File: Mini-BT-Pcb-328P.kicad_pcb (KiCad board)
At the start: 2 copper layers, 55 x 35 mm, 51 parts, among them J1 Analog IN, J2 USB_B_Micro, J3 Booster CE, J5 ANT, P1 MYSX_2.6, Q1 FDN338P, Q2 FDN337N, SW2 Reset, SW3 SW_Reed, U1 ME2188C33, U2 ATSHA204A, U3 AMS1117-3.3, U4 ATmega328P-AU, U5 NRF24L01, U6 NRF24L01, U7 RFM69HW

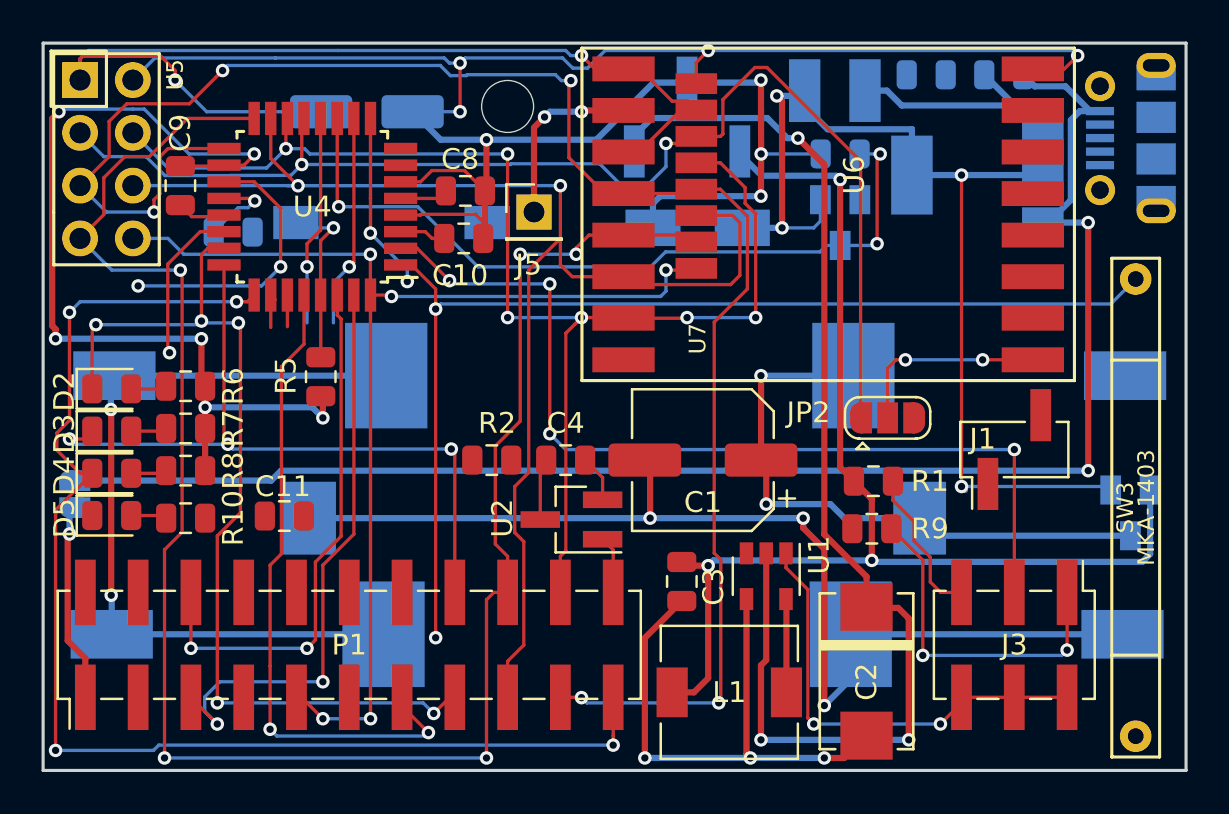
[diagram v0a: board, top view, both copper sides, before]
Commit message: routing test 4
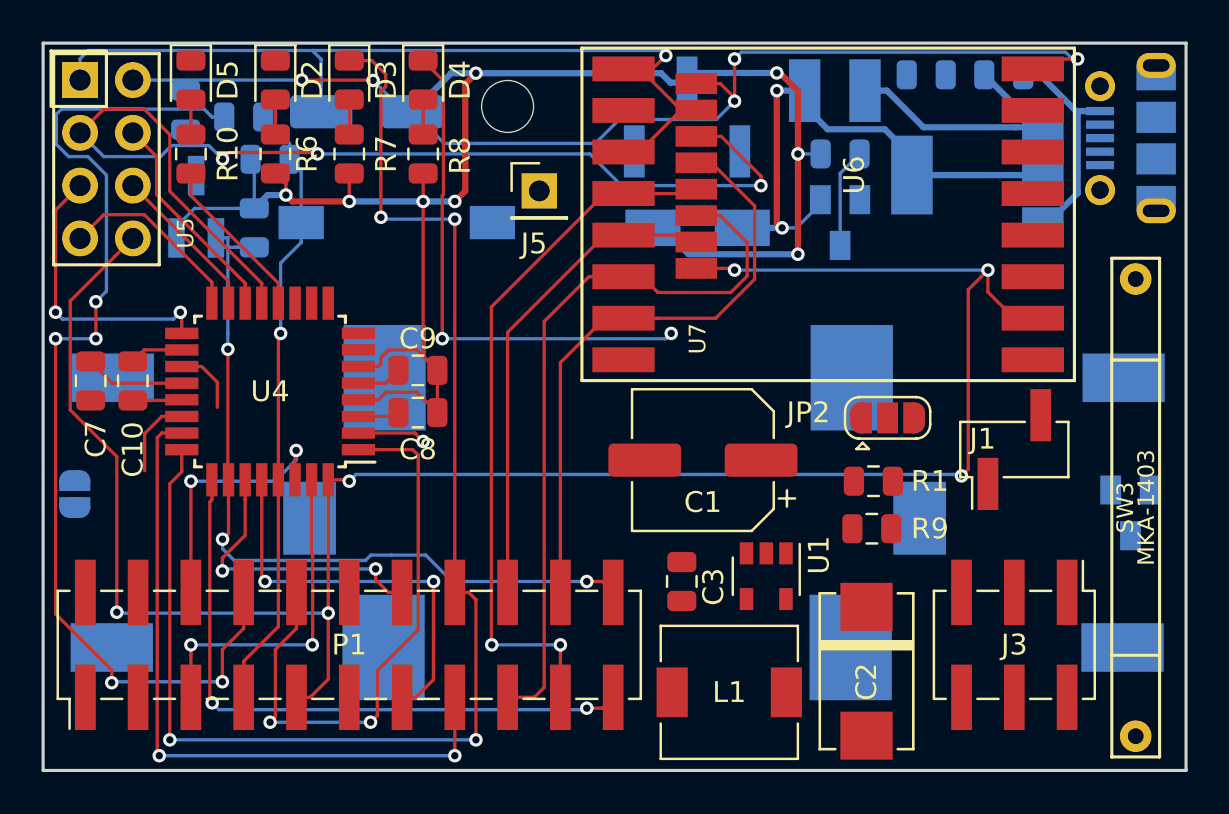
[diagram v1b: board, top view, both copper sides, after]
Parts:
- C11, C4, R2, R5, U2: moved to B.Cu
- C7: moved to F.Cu
- moved C4 24.9 mm to (138.9, 76.6), turned to 90 degrees
- moved D4 24.1 mm to (150.4, 75.2), turned to 270 degrees
- moved U2 23.5 mm to (139.4, 81.3), turned to 90 degrees
- moved D5 21.3 mm to (139.2, 75.2), turned to 270 degrees
- moved D3 20.4 mm to (146.8, 75.2), turned to 270 degrees
- moved C11 19.3 mm to (141.7, 77.0)
- moved R8 19.1 mm to (150.4, 78.7), turned to 270 degrees
- moved R10 17.5 mm to (139.2, 78.7), turned to 270 degrees
- moved C10 17.3 mm to (136.4, 89.7), turned to 90 degrees
- moved D2 16.8 mm to (143.3, 75.2), turned to 270 degrees
- moved R2 16.0 mm to (142.2, 82.3), turned to 270 degrees
- moved R7 15.4 mm to (146.8, 78.7), turned to 270 degrees
- moved C9 14.5 mm to (150.1, 89.2), turned to 0 degrees
- moved R6 12.0 mm to (143.3, 78.7), turned to 270 degrees
- moved C8 10.9 mm to (150.1, 91.2)
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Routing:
- net GND: track 154.0 -> 62.5 mm, vias 8 -> 1
- net Net-(C6-Pad1): track 74.7 -> 10.7 mm, vias 2 -> 0
- net MISO: track 93.1 -> 32.9 mm, vias 5 -> 0
- net Net-(C3-Pad2): track 57.9 -> 0.00 mm, vias 3 -> 0
- net +3.3V: track 57.6 -> 0.00 mm, vias 3 -> 0
- net DTR: track 0.00 -> 50.6 mm, vias 0 -> 5
- net D2: track 55.0 -> 100.8 mm, vias 5 -> 6
- net D4: track 44.6 -> 3.28 mm, vias 4 -> 1
- net Net-(BT2-Pad2): track 38.7 -> 0.00 mm, vias 2 -> 0
- net SCK: track 83.5 -> 48.2 mm, vias 5 -> 4
- net A3: track 4.64 -> 38.5 mm, vias 0 -> 3
- net Ext-Pwr-Sense: track 37.2 -> 4.79 mm, vias 3 -> 0
- net A1: track 35.5 -> 67.4 mm, vias 3 -> 4
- net Net-(BT1-Pad1): track 29.2 -> 0.00 mm, vias 2 -> 0
- net D3: track 53.2 -> 28.4 mm
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
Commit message: routing test 5
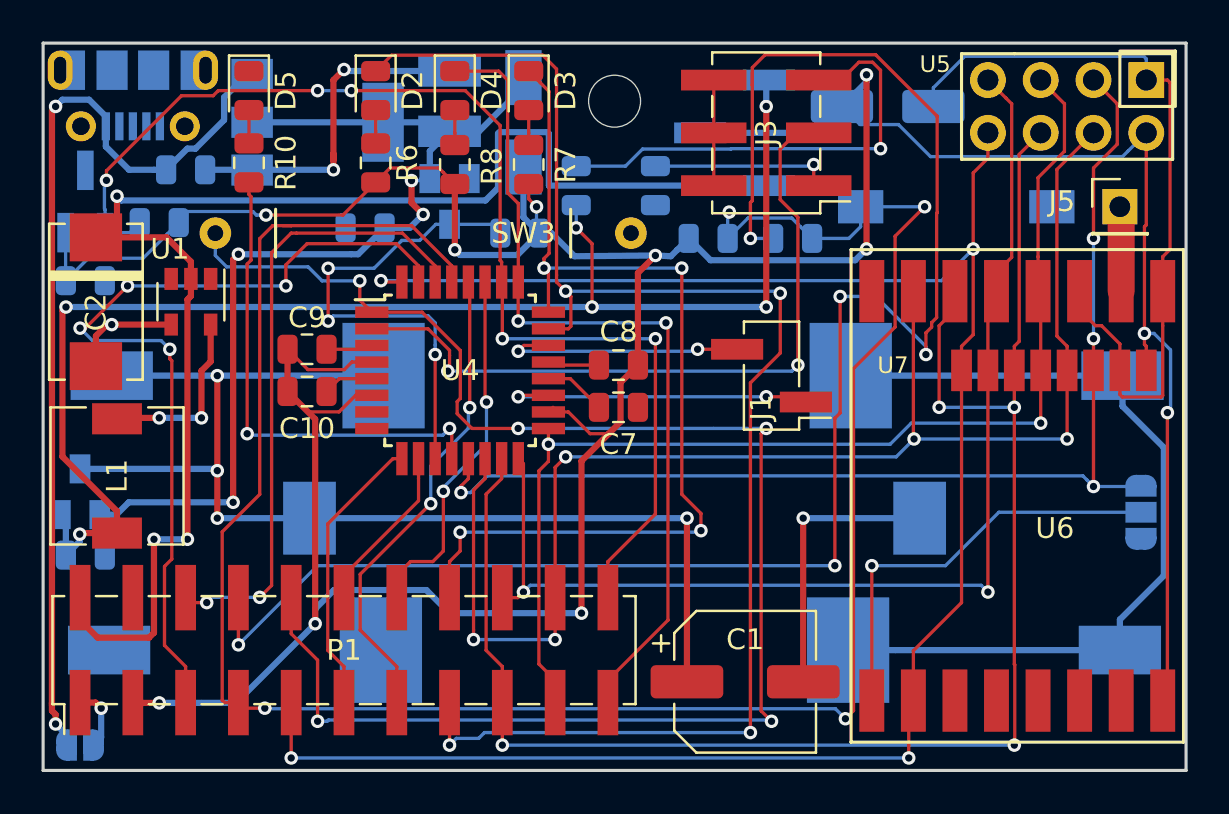
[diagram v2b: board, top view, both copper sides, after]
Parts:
- C3, JP2, R1, R9: moved to B.Cu
- SW3: footprint switches:Reed-MKA-14103-EXT-SILK -> switches:Reed-MKA-14103
- moved U5 54.4 mm to (186.7, 73.7), turned to 0 degrees
- moved Q1 50.6 mm to (133.9, 95.0), turned to 180 degrees
- moved BT2 48.7 mm to (135.4, 89.4), turned to 0 degrees
- moved BT3 48.5 mm to (183.9, 102.6), turned to 180 degrees
- moved J2 48.0 mm to (136.4, 75.9), turned to 0 degrees
- moved C2 41.1 mm to (134.6, 85.9)
- moved C6 39.6 mm to (138.9, 79.5), turned to 0 degrees
- moved SW3 36.7 mm to (150.4, 82.5), turned to 0 degrees
- moved U3 31.9 mm to (145.3, 77.2), turned to 0 degrees
- moved L1 31.3 mm to (135.6, 94.2), turned to 90 degrees
- moved U1 30.7 mm to (139.2, 85.9)
- moved C3 28.7 mm to (134.1, 98.0), turned to 180 degrees
- moved R3 28.0 mm to (147.6, 82.3), turned to 0 degrees
- moved J5 28.0 mm to (183.9, 81.3)
- moved J3 27.4 mm to (166.9, 77.7), turned to 180 degrees
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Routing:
- net RESET: track 29.8 -> 103.8 mm, vias 1 -> 4
- net +3.3V: track 0.00 -> 69.0 mm, vias 0 -> 3
- net Net-(C3-Pad2): track 0.00 -> 68.2 mm, vias 0 -> 6
- net Net-(BT1-Pad1): track 0.00 -> 57.1 mm, vias 0 -> 4
- net VCC: track 141.0 -> 190.2 mm, vias 13 -> 11
- net D3: track 28.4 -> 76.3 mm, vias 2 -> 5
- net Net-(BT2-Pad2): track 0.00 -> 41.1 mm
- net A0: track 33.7 -> 72.2 mm, vias 2 -> 4
- net MOSI: track 43.0 -> 78.7 mm, vias 0 -> 4
- net Net-(C6-Pad1): track 10.7 -> 45.6 mm, vias 0 -> 2
- net DTR: track 50.6 -> 83.1 mm
- net D4: track 3.28 -> 35.1 mm, vias 1 -> 2
- net NSS: track 39.7 -> 69.1 mm, vias 0 -> 5
- net Net-(C5-Pad1): track 26.6 -> 51.7 mm, vias 2 -> 4
- net D1-TXD: track 17.4 -> 42.1 mm, vias 2 -> 4
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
